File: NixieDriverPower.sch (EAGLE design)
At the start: 18 parts, among them IC1 MC34063AD, T1 MJD31

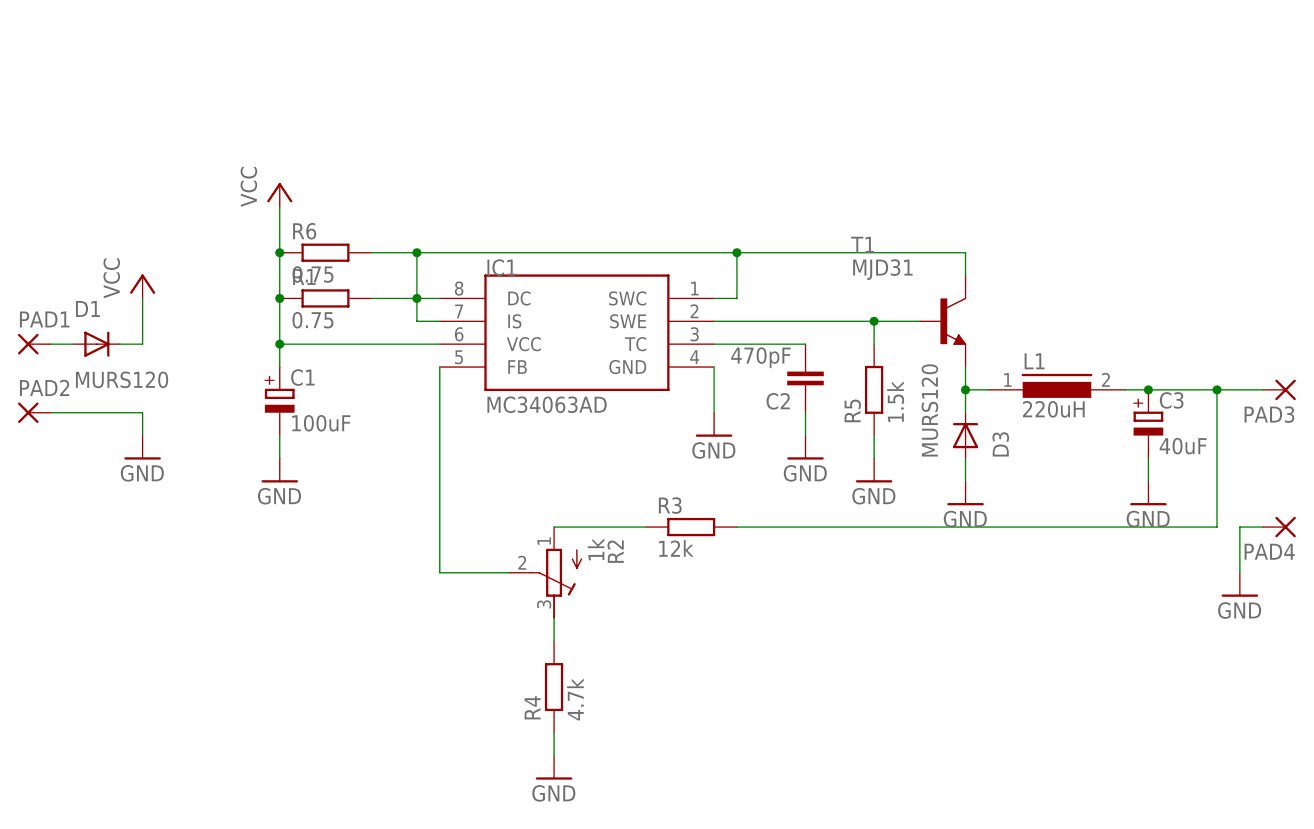
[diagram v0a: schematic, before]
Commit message: Commit of the current version
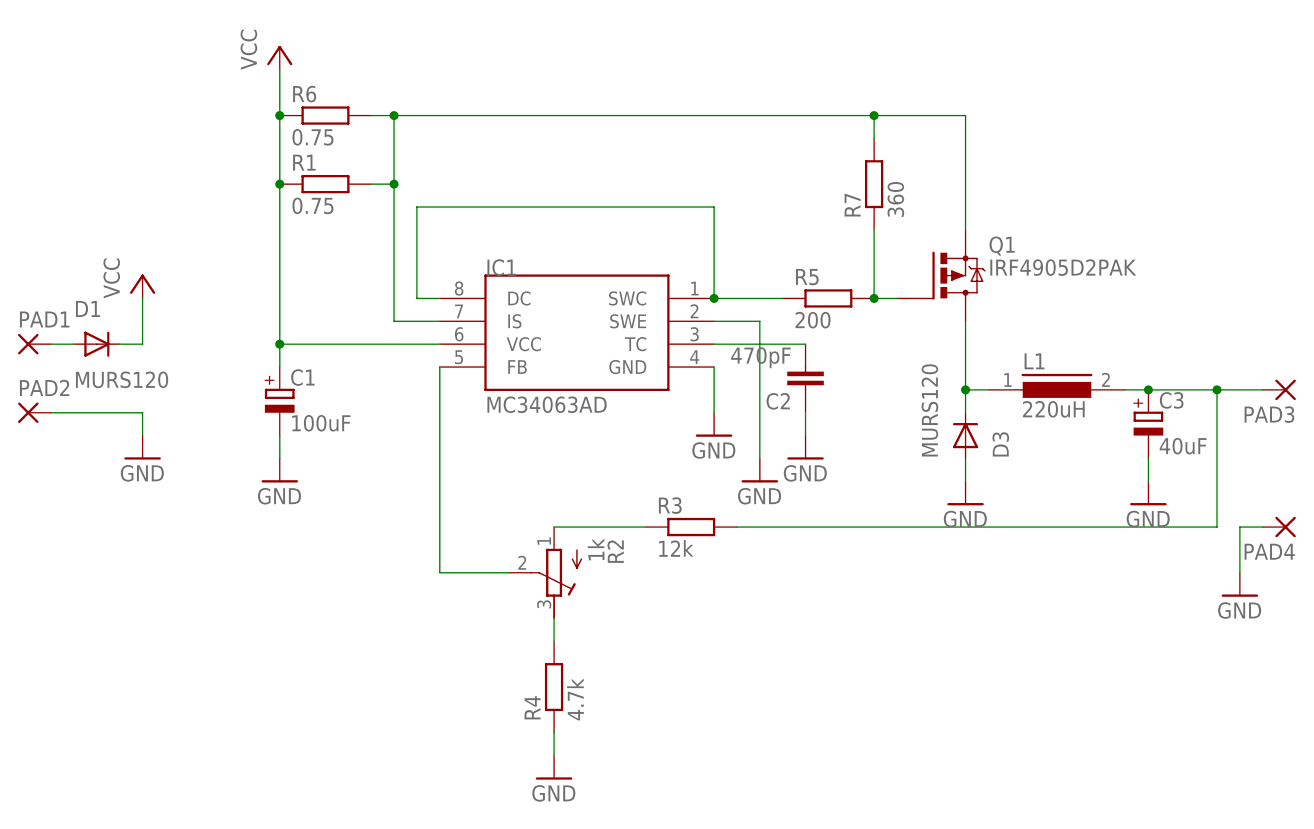
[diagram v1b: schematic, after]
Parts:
- removed T1: MJD31, transistor:MJD31
- added Q1: IRF4905D2PAK, own-collection:IRF4905D2PAK
- added R7: 360, rcl-2:R-EU_R1206
- R5: value 1.5k -> 200
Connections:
- removed net N$3: IC1.DC, IC1.IS, IC1.SWC, R1.2, R6.2, T1.C
- new net N$10: IC1.DC, IC1.SWC, R5.1
- new net N$5: IC1.IS, Q1.S, R1.2, R6.2, R7.2
- net GND: now also IC1.SWE; no longer R5.1
- net N$1: now also Q1.D; no longer T1.E
- net N$4: now also Q1.G, R7.1; no longer IC1.SWE, T1.B
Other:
- moved on the sheet: R1, R5, R6
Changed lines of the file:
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@@
 <part name="R2" library="rcl" deviceset="R-TRIMM" device="4G/J" value="1k"/>
 <part name="D1" library="diode" deviceset="DIODE-" device="DO214AA" value="MURS120"/>
-<part name="T1" library="transistor" deviceset="MJD31*" device=""/>
 <part name="GND9" library="supply1" deviceset="GND" device=""/>
-<part name="R5" library="rcl-2" deviceset="R-EU_" device="R1206" value="1.5k"/>
-<part name="GND10" library="supply1" deviceset="GND" device=""/>
+<part name="Q1" library="own-collection" deviceset="IRF4905" device="D2PAK"/>
+<part name="R5" library="rcl-2" deviceset="R-EU_" device="R1206" value="200"/>
+<part name="R7" library="rcl-2" deviceset="R-EU_" device="R1206" value="360"/>
+<part name="GND8" library="supply1" deviceset="GND" device=""/>
 </parts>
 <sheets>
@@
 <instance part="IC1" gate="G$1" x="68.58" y="60.96"/>
 <instance part="L1" gate="G$1" x="121.92" y="50.8"/>
-<instance part="R1" gate="G$1" x="40.64" y="60.96"/>
+<instance part="R1" gate="G$1" x="40.64" y="73.66"/>
 <instance part="C1" gate="G$1" x="35.56" y="50.8"/>
 <instance part="GND1" gate="1" x="35.56" y="40.64"/>
@@
 <attribute name="VALUE" x="106.9086" y="43.18" size="1.778" layer="96" rot="MR90"/>
 </instance>
-<instance part="R6" gate="G$1" x="40.64" y="66.04"/>
-<instance part="P+1" gate="VCC" x="35.56" y="73.66"/>
+<instance part="R6" gate="G$1" x="40.64" y="81.28"/>
+<instance part="P+1" gate="VCC" x="35.56" y="88.9"/>
 <instance part="P+5" gate="VCC" x="20.32" y="63.5"/>
 <instance part="R2" gate="G$1" x="66.04" y="30.48" rot="R180"/>
@@
 <attribute name="VALUE" x="12.7" y="51.0286" size="1.778" layer="96"/>
 </instance>
-<instance part="T1" gate="G$1" x="109.22" y="58.42"/>
 <instance part="GND9" gate="1" x="111.76" y="38.1"/>
-<instance part="R5" gate="G$1" x="101.6" y="50.8" rot="R90"/>
-<instance part="GND10" gate="1" x="101.6" y="40.64"/>
+<instance part="Q1" gate="G$1" x="109.22" y="63.5"/>
+<instance part="R5" gate="G$1" x="96.52" y="60.96"/>
+<instance part="R7" gate="G$1" x="101.6" y="73.66" rot="R90"/>
+<instance part="GND8" gate="1" x="88.9" y="40.64"/>
 </instances>
 <busses>
 </busses>
 <nets>
-<net name="N$3" class="0">
-<segment>
-<pinref part="R6" gate="G$1" pin="2"/>
-<wire x1="45.72" y1="66.04" x2="50.8" y2="66.04" width="0.1524" layer="91"/>
-<pinref part="IC1" gate="G$1" pin="DC"/>
-<wire x1="53.34" y1="60.96" x2="50.8" y2="60.96" width="0.1524" layer="91"/>
-<wire x1="50.8" y1="60.96" x2="50.8" y2="66.04" width="0.1524" layer="91"/>
-<wire x1="50.8" y1="66.04" x2="86.36" y2="66.04" width="0.1524" layer="91"/>
-<wire x1="86.36" y1="66.04" x2="86.36" y2="60.96" width="0.1524" layer="91"/>
-<pinref part="IC1" gate="G$1" pin="SWC"/>
-<wire x1="86.36" y1="60.96" x2="83.82" y2="60.96" width="0.1524" layer="91"/>
-<pinref part="IC1" gate="G$1" pin="IS"/>
-<wire x1="50.8" y1="60.96" x2="50.8" y2="58.42" width="0.1524" layer="91"/>
-<wire x1="50.8" y1="58.42" x2="53.34" y2="58.42" width="0.1524" layer="91"/>
-<junction x="50.8" y="60.96"/>
-<junction x="50.8" y="66.04"/>
-<wire x1="86.36" y1="66.04" x2="111.76" y2="66.04" width="0.1524" layer="91"/>
-<wire x1="111.76" y1="66.04" x2="111.76" y2="63.5" width="0.1524" layer="91"/>
-<junction x="86.36" y="66.04"/>
-<pinref part="T1" gate="G$1" pin="C"/>
-<pinref part="R1" gate="G$1" pin="2"/>
-<wire x1="45.72" y1="60.96" x2="50.8" y2="60.96" width="0.1524" layer="91"/>
-</segment>
-</net>
 <net name="GND" class="0">
 <segment>
@@
 </segment>
 <segment>
-<pinref part="R5" gate="G$1" pin="1"/>
-<wire x1="101.6" y1="45.72" x2="101.6" y2="43.18" width="0.1524" layer="91"/>
-<pinref part="GND10" gate="1" pin="GND"/>
+<wire x1="88.9" y1="58.42" x2="88.9" y2="43.18" width="0.1524" layer="91"/>
+<pinref part="GND8" gate="1" pin="GND"/>
+<pinref part="IC1" gate="G$1" pin="SWE"/>
+<wire x1="83.82" y1="58.42" x2="88.9" y2="58.42" width="0.1524" layer="91"/>
 </segment>
 </net>
@@
 <wire x1="53.34" y1="30.48" x2="53.34" y2="53.34" width="0.1524" layer="91"/>
 <pinref part="R2" gate="G$1" pin="S"/>
-<wire x1="60.96" y1="30.48" x2="53.34" y2="30.48" width="0.1524" layer="91"/>
+<wire x1="53.34" y1="30.48" x2="60.96" y2="30.48" width="0.1524" layer="91"/>
 </segment>
 </net>
@@
 <segment>
 <pinref part="R1" gate="G$1" pin="1"/>
-<wire x1="35.56" y1="60.96" x2="35.56" y2="55.88" width="0.1524" layer="91"/>
+<wire x1="35.56" y1="73.66" x2="35.56" y2="55.88" width="0.1524" layer="91"/>
 <pinref part="C1" gate="G$1" pin="+"/>
 <pinref part="R6" gate="G$1" pin="1"/>
 <wire x1="35.56" y1="55.88" x2="35.56" y2="53.34" width="0.1524" layer="91"/>
-<wire x1="35.56" y1="66.04" x2="35.56" y2="60.96" width="0.1524" layer="91"/>
-<junction x="35.56" y="60.96"/>
+<wire x1="35.56" y1="81.28" x2="35.56" y2="73.66" width="0.1524" layer="91"/>
+<junction x="35.56" y="73.66"/>
 <pinref part="P+1" gate="VCC" pin="VCC"/>
-<wire x1="35.56" y1="66.04" x2="35.56" y2="71.12" width="0.1524" layer="91"/>
-<junction x="35.56" y="66.04"/>
+<wire x1="35.56" y1="81.28" x2="35.56" y2="86.36" width="0.1524" layer="91"/>
+<junction x="35.56" y="81.28"/>
 <pinref part="IC1" gate="G$1" pin="VCC"/>
 <wire x1="53.34" y1="55.88" x2="35.56" y2="55.88" width="0.1524" layer="91"/>
@@
 </segment>
 </net>
-<net name="N$9" class="0">
-<segment>
-<pinref part="R2" gate="G$1" pin="A"/>
-<pinref part="R3" gate="G$1" pin="1"/>
-<wire x1="66.04" y1="35.56" x2="76.2" y2="35.56" width="0.1524" layer="91"/>
-</segment>
-</net>
-<net name="N$10" class="0">
-<segment>
-<pinref part="R2" gate="G$1" pin="E"/>
-<pinref part="R4" gate="G$1" pin="2"/>
-<wire x1="66.04" y1="25.4" x2="66.04" y2="22.86" width="0.1524" layer="91"/>
-</segment>
-</net>
 <net name="N$12" class="0">
 <segment>
@@
 </segment>
 </net>
-<net name="N$4" class="0">
-<segment>
-<pinref part="IC1" gate="G$1" pin="SWE"/>
-<pinref part="T1" gate="G$1" pin="B"/>
-<wire x1="83.82" y1="58.42" x2="101.6" y2="58.42" width="0.1524" layer="91"/>
-<pinref part="R5" gate="G$1" pin="2"/>
-<wire x1="101.6" y1="58.42" x2="106.68" y2="58.42" width="0.1524" layer="91"/>
-<wire x1="101.6" y1="55.88" x2="101.6" y2="58.42" width="0.1524" layer="91"/>
-<junction x="101.6" y="58.42"/>
-</segment>
-</net>
 <net name="N$1" class="0">
 <segment>
-<pinref part="T1" gate="G$1" pin="E"/>
 <pinref part="D3" gate="G$1" pin="C"/>
-<wire x1="111.76" y1="53.34" x2="111.76" y2="50.8" width="0.1524" layer="91"/>
 <pinref part="L1" gate="G$1" pin="1"/>
 <wire x1="111.76" y1="50.8" x2="111.76" y2="48.26" width="0.1524" layer="91"/>
 <wire x1="111.76" y1="50.8" x2="114.3" y2="50.8" width="0.1524" layer="91"/>
 <junction x="111.76" y="50.8"/>
-</segment>
-</net>
+<pinref part="Q1" gate="G$1" pin="D"/>
+<wire x1="111.76" y1="58.42" x2="111.76" y2="50.8" width="0.1524" layer="91"/>
+</segment>
+</net>
+<net name="N$5" class="0">
+<segment>
+<pinref part="R6" gate="G$1" pin="2"/>
+<wire x1="45.72" y1="81.28" x2="48.26" y2="81.28" width="0.1524" layer="91"/>
+<pinref part="R1" gate="G$1" pin="2"/>
+<wire x1="45.72" y1="73.66" x2="48.26" y2="73.66" width="0.1524" layer="91"/>
+<wire x1="48.26" y1="81.28" x2="48.26" y2="73.66" width="0.1524" layer="91"/>
+<pinref part="IC1" gate="G$1" pin="IS"/>
+<wire x1="48.26" y1="73.66" x2="48.26" y2="58.42" width="0.1524" layer="91"/>
+<wire x1="48.26" y1="58.42" x2="53.34" y2="58.42" width="0.1524" layer="91"/>
+<junction x="48.26" y="73.66"/>
+<junction x="48.26" y="81.28"/>
+<pinref part="R7" gate="G$1" pin="2"/>
+<wire x1="48.26" y1="81.28" x2="101.6" y2="81.28" width="0.1524" layer="91"/>
+<wire x1="101.6" y1="81.28" x2="101.6" y2="78.74" width="0.1524" layer="91"/>
+<pinref part="Q1" gate="G$1" pin="S"/>
+<wire x1="101.6" y1="81.28" x2="111.76" y2="81.28" width="0.1524" layer="91"/>
+<wire x1="111.76" y1="81.28" x2="111.76" y2="68.58" width="0.1524" layer="91"/>
+<junction x="101.6" y="81.28"/>
+</segment>
+</net>
+<net name="N$4" class="0">
+<segment>
+<pinref part="Q1" gate="G$1" pin="G"/>
+<pinref part="R5" gate="G$1" pin="2"/>
+<wire x1="101.6" y1="60.96" x2="104.14" y2="60.96" width="0.1524" layer="91"/>
+<wire x1="101.6" y1="68.58" x2="101.6" y2="60.96" width="0.1524" layer="91"/>
+<junction x="101.6" y="60.96"/>
+<pinref part="R7" gate="G$1" pin="1"/>
+</segment>
+</net>
+<net name="N$10" class="0">
+<segment>
+<pinref part="IC1" gate="G$1" pin="DC"/>
+<wire x1="53.34" y1="60.96" x2="50.8" y2="60.96" width="0.1524" layer="91"/>
+<wire x1="50.8" y1="60.96" x2="50.8" y2="71.12" width="0.1524" layer="91"/>
+<wire x1="50.8" y1="71.12" x2="83.82" y2="71.12" width="0.1524" layer="91"/>
+<pinref part="R5" gate="G$1" pin="1"/>
+<pinref part="IC1" gate="G$1" pin="SWC"/>
+<wire x1="83.82" y1="60.96" x2="91.44" y2="60.96" width="0.1524" layer="91"/>
+<wire x1="83.82" y1="60.96" x2="83.82" y2="71.12" width="0.1524" layer="91"/>
+<junction x="83.82" y="60.96"/>
+</segment>
+</net>
+<net name="N$8" class="0">
+<segment>
+<pinref part="R2" gate="G$1" pin="E"/>
+<pinref part="R4" gate="G$1" pin="2"/>
+<wire x1="66.04" y1="25.4" x2="66.04" y2="22.86" width="0.1524" layer="91"/>
+</segment>
+</net>
+<net name="N$9" class="0">
+<segment>
+<pinref part="R2" gate="G$1" pin="A"/>
+<pinref part="R3" gate="G$1" pin="1"/>
+<wire x1="66.04" y1="35.56" x2="76.2" y2="35.56" width="0.1524" layer="91"/>
+</segment>
+</net>
